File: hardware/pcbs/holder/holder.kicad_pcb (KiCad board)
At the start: 2 copper layers, 80 x 50.5 mm, 0 parts

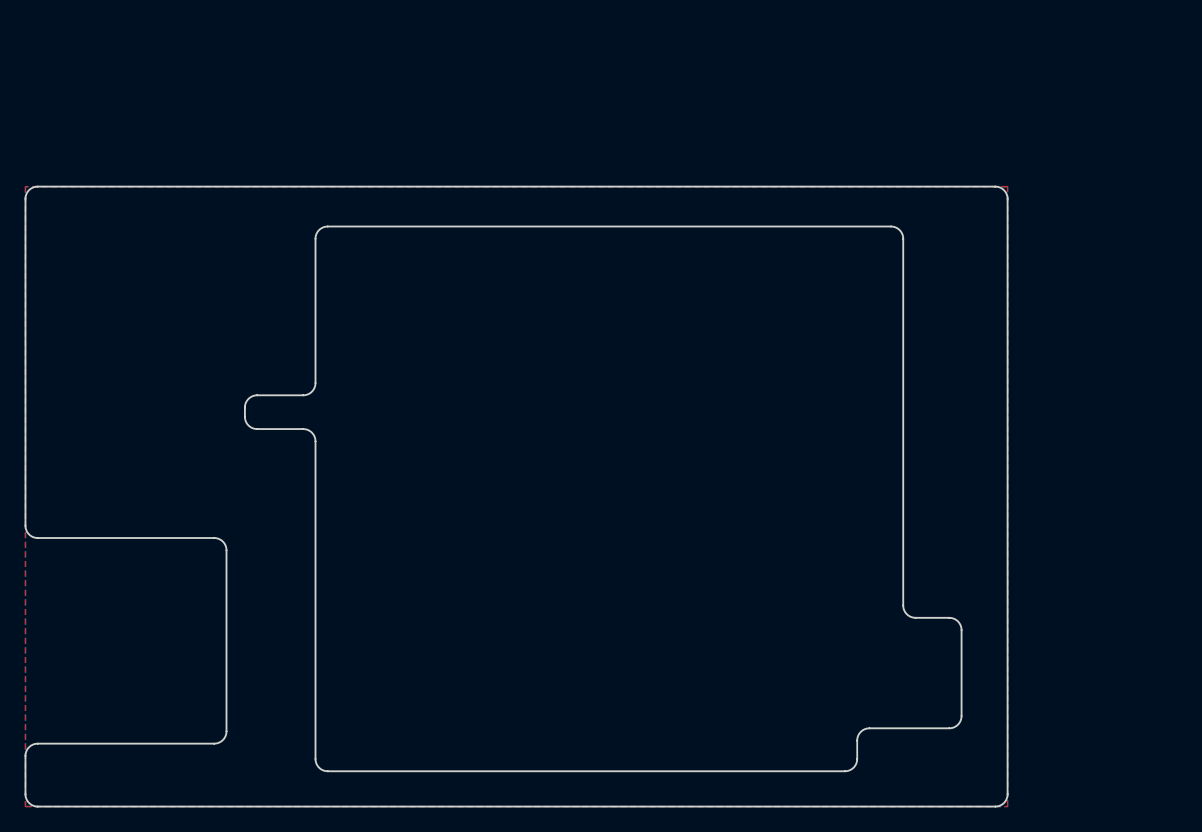
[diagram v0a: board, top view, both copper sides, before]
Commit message: chore: finalize v6c production run
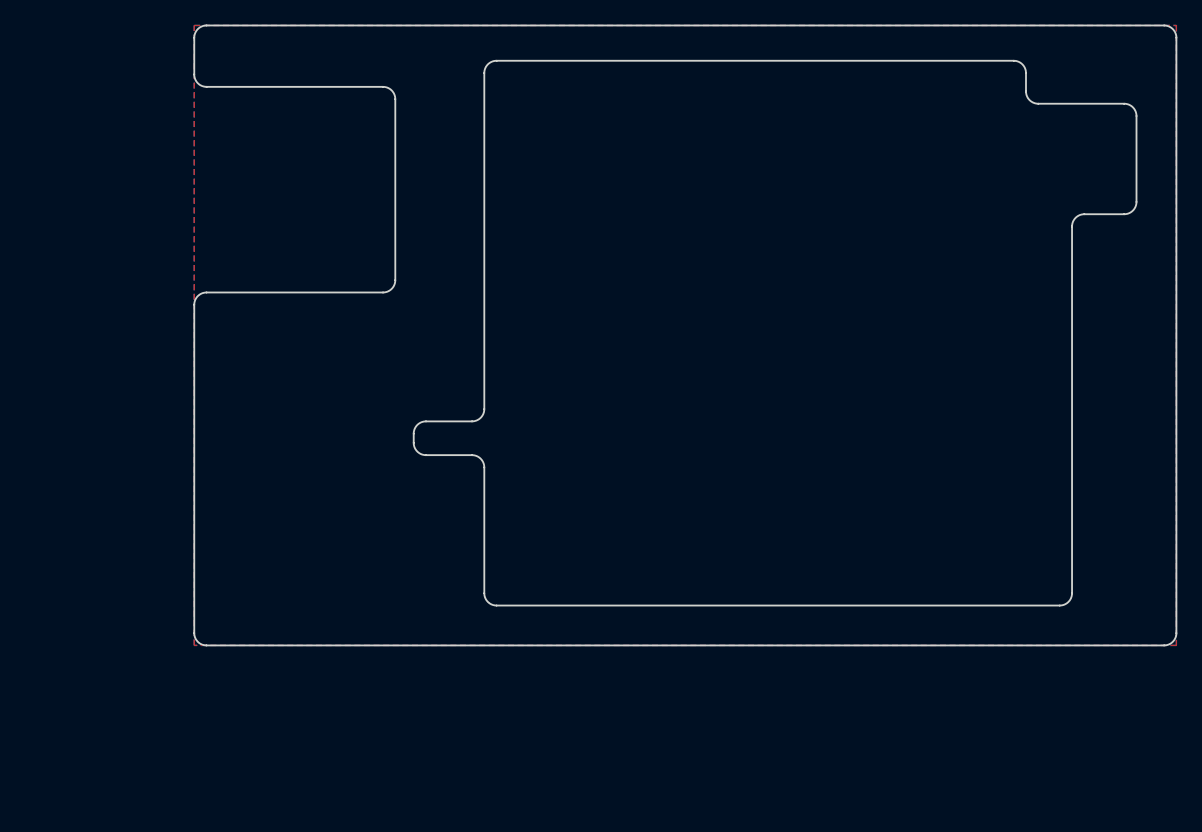
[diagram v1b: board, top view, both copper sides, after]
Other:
- outline, holes or cut-outs redrawn
